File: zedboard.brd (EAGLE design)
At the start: 150 x 100 mm, 24 parts, among them U1 A540Q, U1_C1 0.1u, U1_C2 0.1u

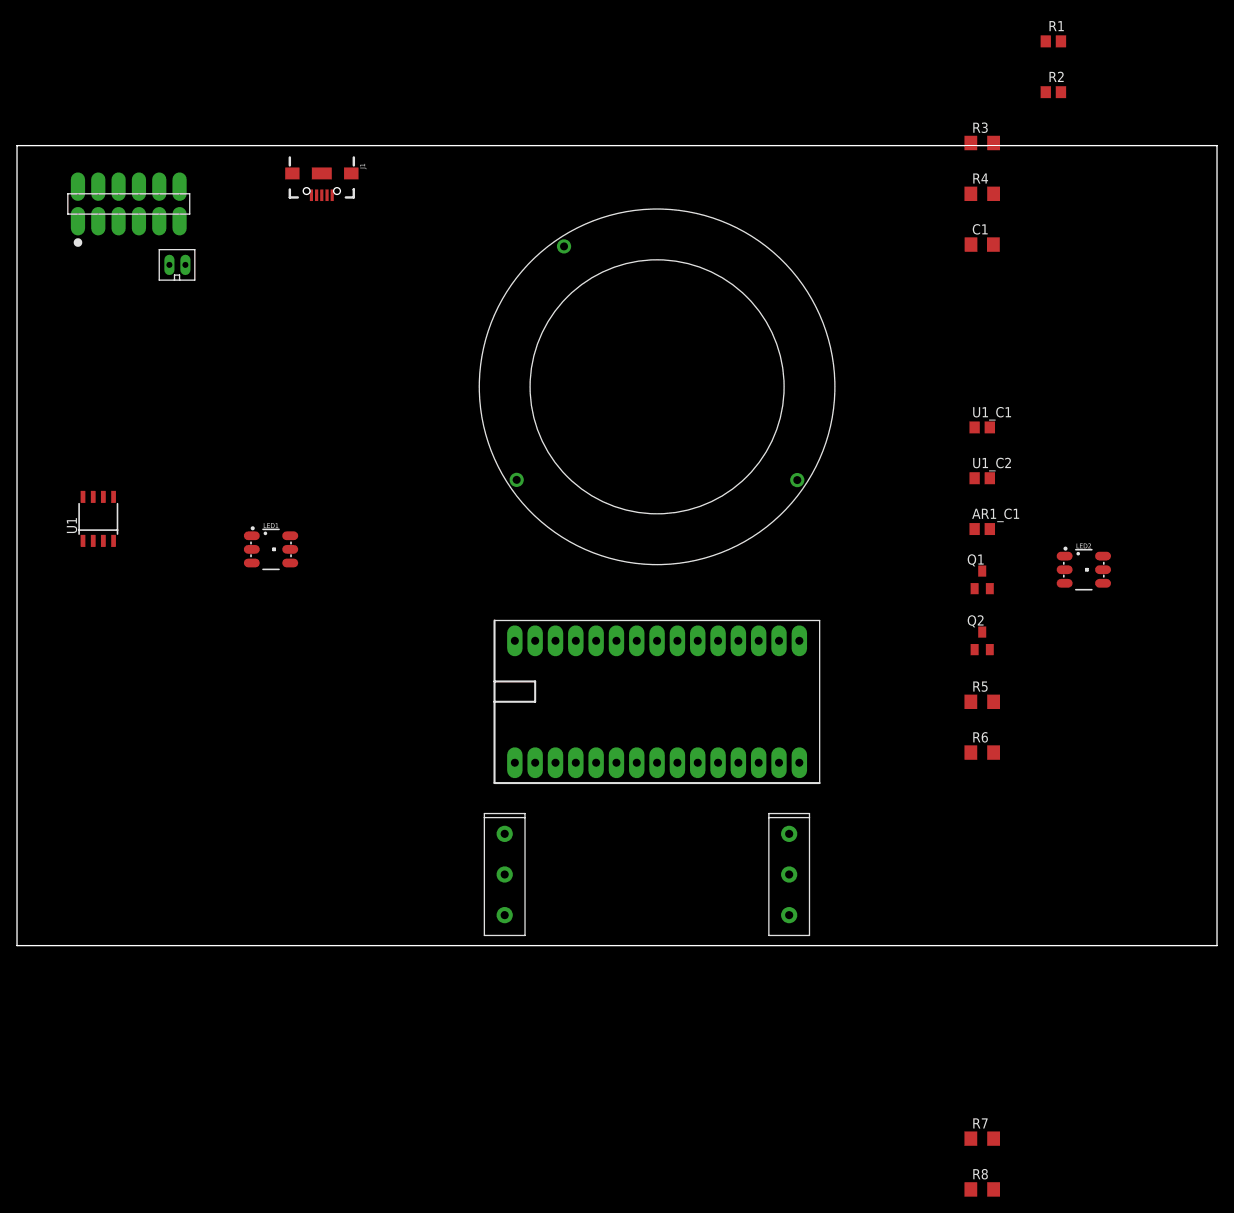
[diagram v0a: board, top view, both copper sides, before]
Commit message: finish design
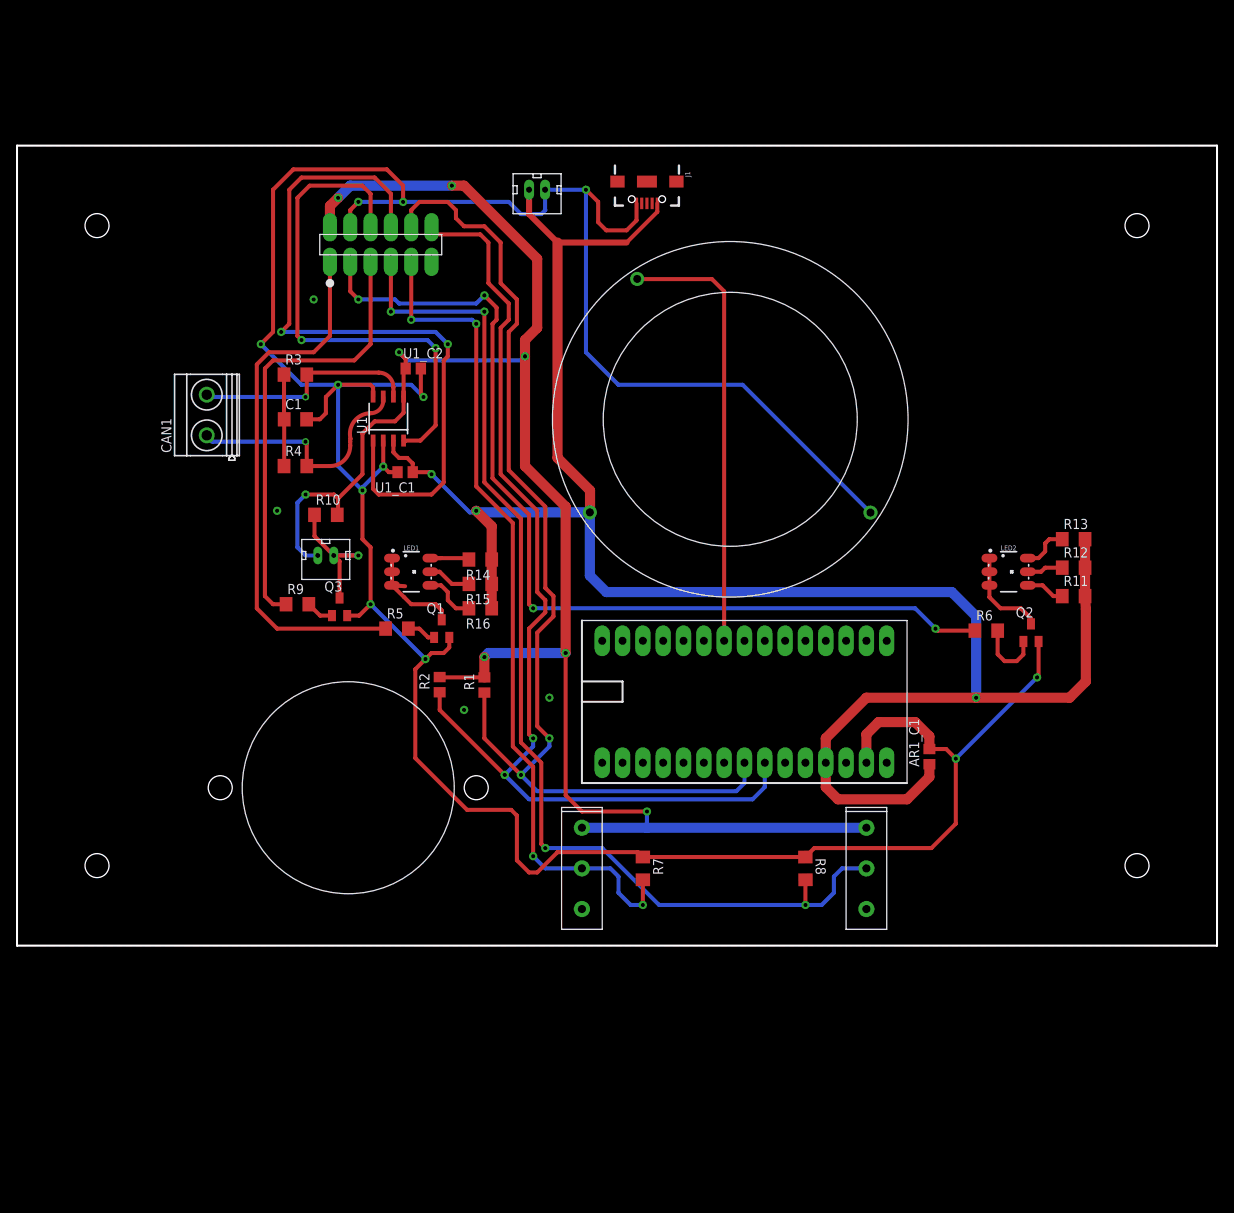
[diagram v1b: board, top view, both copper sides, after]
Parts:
- removed J$3: HEARDER_2X1, connectors:HEARDER_2X1_2MM
- added CAN1: MKDSN1,5/2-5,08, con-phoenix-508:MKDSN1,5/2-5,08
- added JST1: USB5V, Justin-Eagle-Lib:POWER_2MM
- added Q3: BC547, semicon-smd-ipc:SOT23
- added R10, R9: 1K, rcl:R1206
- added R11, R12, R13, R14, R15, R16: 220, rcl:R1206
- added SP1: DC-3V, Justin-Eagle-Lib:SPEAKER_2MM_CON
- AR1_C1: value (none) -> 0.1u
- J1: value (none) -> Micro-USB
- Q1, Q2: value (none) -> BC547
- R7, R8: value (none) -> 220
- SW1, SW2: value (none) -> 1A125V
- moved R1 107.4 mm to (58.4, 32.6), turned to 90 degrees
- moved R2 106.6 mm to (52.8, 32.6), turned to 90 degrees
- moved R4 92.4 mm to (34.8, 59.9)
- moved R3 90.6 mm to (34.8, 71.4)
- moved C1 88.6 mm to (34.8, 65.8)
- moved R5 73.7 mm to (47.5, 39.6)
- moved U1_C2 72.4 mm to (49.5, 72.1)
- moved U1_C1 72.4 mm to (48.5, 59.2), turned to 180 degrees
- moved Q1 67.8 mm to (53.1, 39.6)
- moved R7 54.2 mm to (78.2, 9.65), turned to 270 degrees
- moved R8 45.8 mm to (98.6, 9.65), turned to 270.4 degrees
- moved J1 40.7 mm to (78.7, 95.5)
- moved U1 38.4 mm to (46.4, 65.9)
- moved U$2 31.9 mm to (39.1, 86.4)
- moved AR1_C1 29.2 mm to (114.0, 23.6), turned to 90 degrees
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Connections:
- removed net N$6: U$2.6
- new net N$10: LED1.5, R15.2
- new net N$11: LED1.6, R14.2
- new net N$12: LED2.4, R11.1
- new net N$13: LED2.5, R12.1
- new net N$14: LED2.6, R13.1
- new net N$7: Q3.3, R10.1, SP1.P$2
- new net N$8: Q3.1, R9.2
- new net N$9: LED1.4, R16.2
- net 3.3V: now also R10.2, SP1.P$1
- net 5V: now also JST1.1, R11.2, R12.2, R13.2, R14.1, R15.1, R16.1; no longer J$3.1, LED1.4, LED1.5, LED1.6, LED2.4, LED2.5, LED2.6
- net CAN_H: now also CAN1.1
- net CAN_L: now also CAN1.2
- net GND: now also JST1.2, Q3.2; no longer J$3.2
- net SP: now also R9.1
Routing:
- net GND: track 0.00 -> 387.0 mm, vias 0 -> 16
- net 5V: track 0.00 -> 245.8 mm, vias 0 -> 3
- net 3.3V: track 0.00 -> 227.5 mm, vias 0 -> 8
- net SW_L: track 0.00 -> 138.3 mm, vias 0 -> 4
- net SDA: track 0.00 -> 134.3 mm, vias 0 -> 2
- net SCL: track 0.00 -> 131.5 mm, vias 0 -> 2
- net LED_R: track 0.00 -> 120.8 mm, vias 0 -> 4
- net SW_R: track 0.00 -> 106.5 mm, vias 0 -> 4
- net CAN_TX: track 0.00 -> 92.2 mm, vias 0 -> 2
- net LED_L: track 0.00 -> 68.4 mm
- net CAN_RX: track 0.00 -> 65.1 mm, vias 0 -> 2
- net SP: track 0.00 -> 57.2 mm
- net NEO_SIG: track 0.00 -> 55.2 mm
- net CAN_H: track 0.00 -> 30.0 mm, vias 0 -> 1
- net CAN_L: track 0.00 -> 28.2 mm, vias 0 -> 1
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- added copper zone on layer 1, net GND
- added copper zone on layer 16, net GND
